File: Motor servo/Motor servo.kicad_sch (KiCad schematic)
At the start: 3 parts

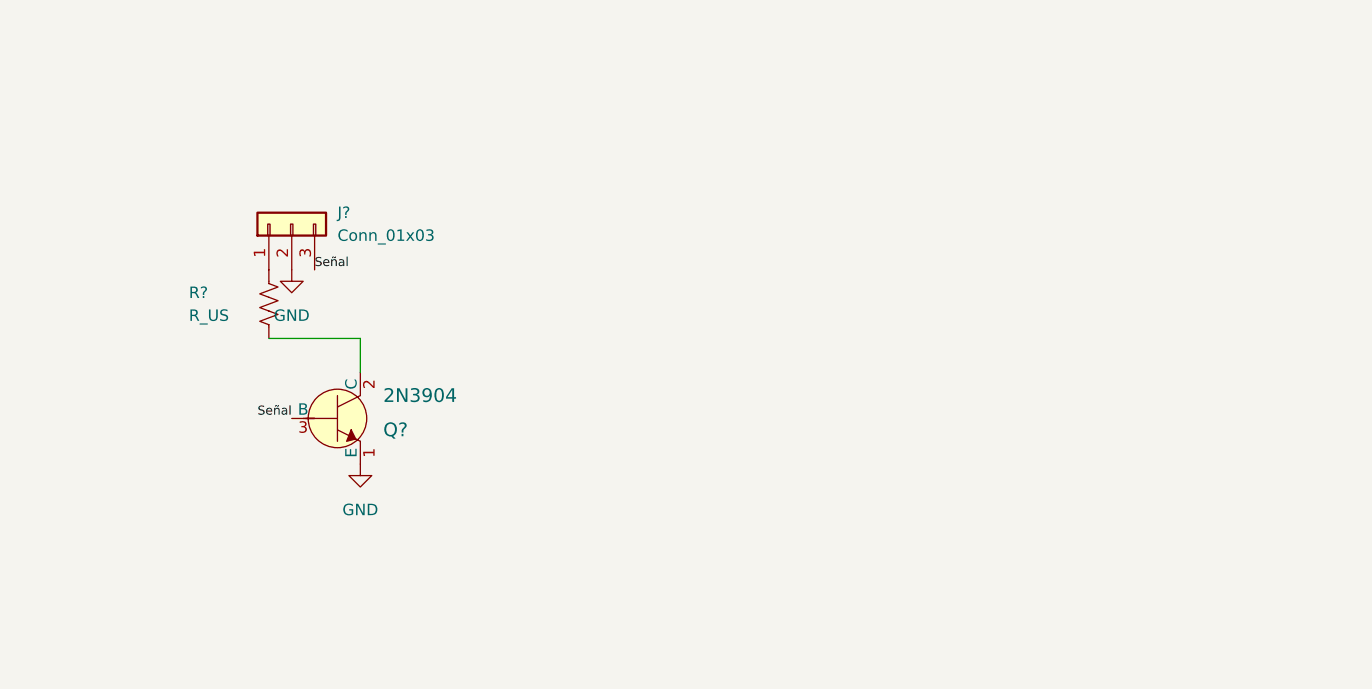
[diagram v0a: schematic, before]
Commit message: final
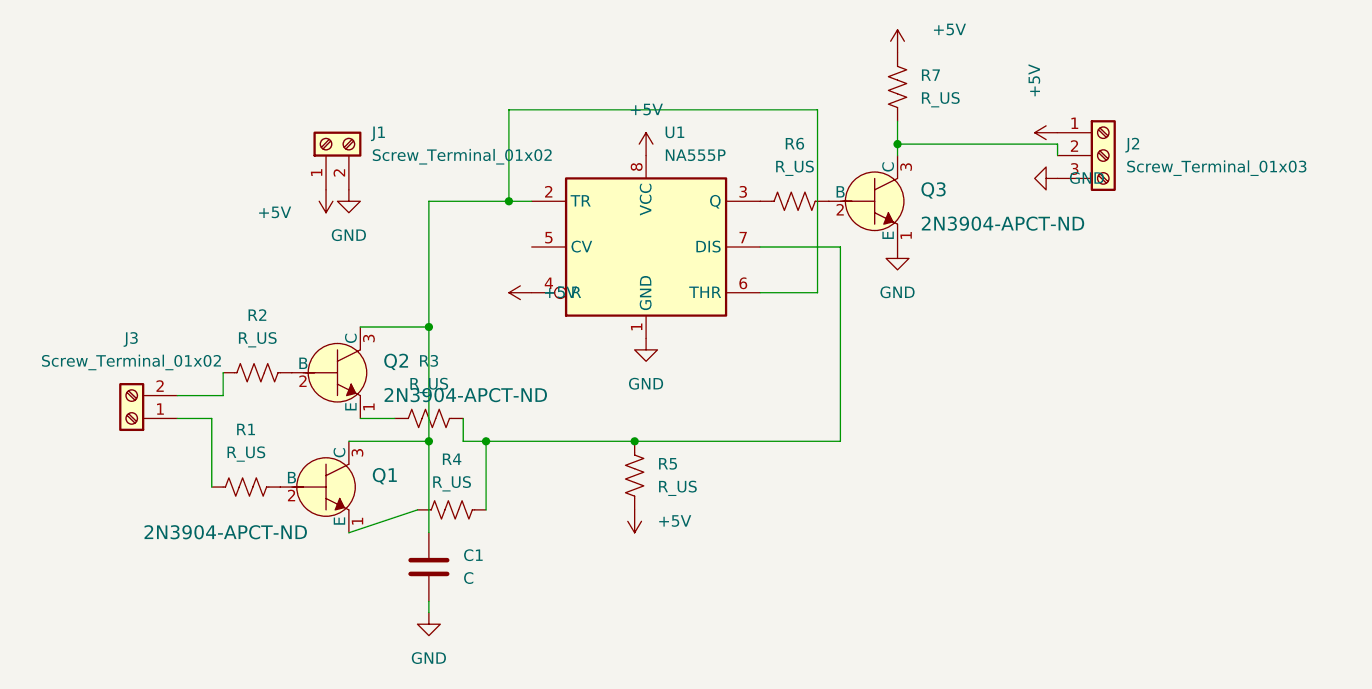
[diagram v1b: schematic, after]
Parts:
- removed J?: Conn_01x03, symbol Connector_Generic:Conn_01x03
- removed Q?: 2N3904, digikey-footprints:TO-92-3, symbol dk_Transistors-Bipolar-BJT-Single:2N3904
- removed R?: R_US, symbol Device:R_US
- added C1: C, Capacitor_THT:C_Disc_D3.0mm_W1.6mm_P2.50mm, symbol Device:C
- added J1, J3: Screw_Terminal_01x02, TerminalBlock:TerminalBlock_bornier-2_P5.08mm, symbol Connector:Screw_Terminal_01x02
- added J2: Screw_Terminal_01x03, TerminalBlock:TerminalBlock_bornier-3_P5.08mm, symbol Connector:Screw_Terminal_01x03
- added Q1, Q2, Q3: 2N3904-APCT-ND, Package_TO_SOT_THT:TO-92, symbol 2N3904-APCT-ND:2N3904-APCT-ND
- added R1, R2, R3, R4, R5, R6, R7: R_US, Resistor_THT:R_Axial_DIN0204_L3.6mm_D1.6mm_P5.08mm_Horizontal, symbol Device:R_US
- added U1: NA555P, Package_DIP:DIP-8_W7.62mm, symbol Timer:NA555P
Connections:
- net GND: now also C1.2, J1.2 (Pin_2), J2.3 (Pin_3), Q3.1 (E), U1.1 (GND)
- new net: Q1.1 (E), R4.1
- new net: R3.2, R4.2, R5.1, U1.7 (DIS)
- new net: J2.2 (Pin_2), Q3.3 (C), R7.2
- new net: Q3.2 (B), R6.2
- new net: C1.1, Q1.3 (C), Q2.3 (C), U1.2 (TR), U1.6 (THR)
- new net: Q2.1 (E), R3.1
- new net: Q2.2 (B), R2.2
- new net: Q1.2 (B), R1.2
- new net: R6.1, U1.3 (Q)
- new net: J3.2 (Pin_2), R2.1
- new net: J3.1 (Pin_1), R1.1
- new net +5V: J1.1 (Pin_1), J2.1 (Pin_1), R5.2, R7.1, U1.4 (R), U1.8 (VCC)
